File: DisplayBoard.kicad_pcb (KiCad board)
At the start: 4 copper layers, 35.6 x 38.1 mm, 42 parts, among them J201 Conn_Coaxial, J301 Conn_01x12_Pin, J401 Conn_01x04, Q301 L2N7002SLLT1G, U201 ESP32-S3-PICO-1-N8R2, U401 SN65HVD232, U501 USBLC6-2SC6, U502 AMS1117-3.3

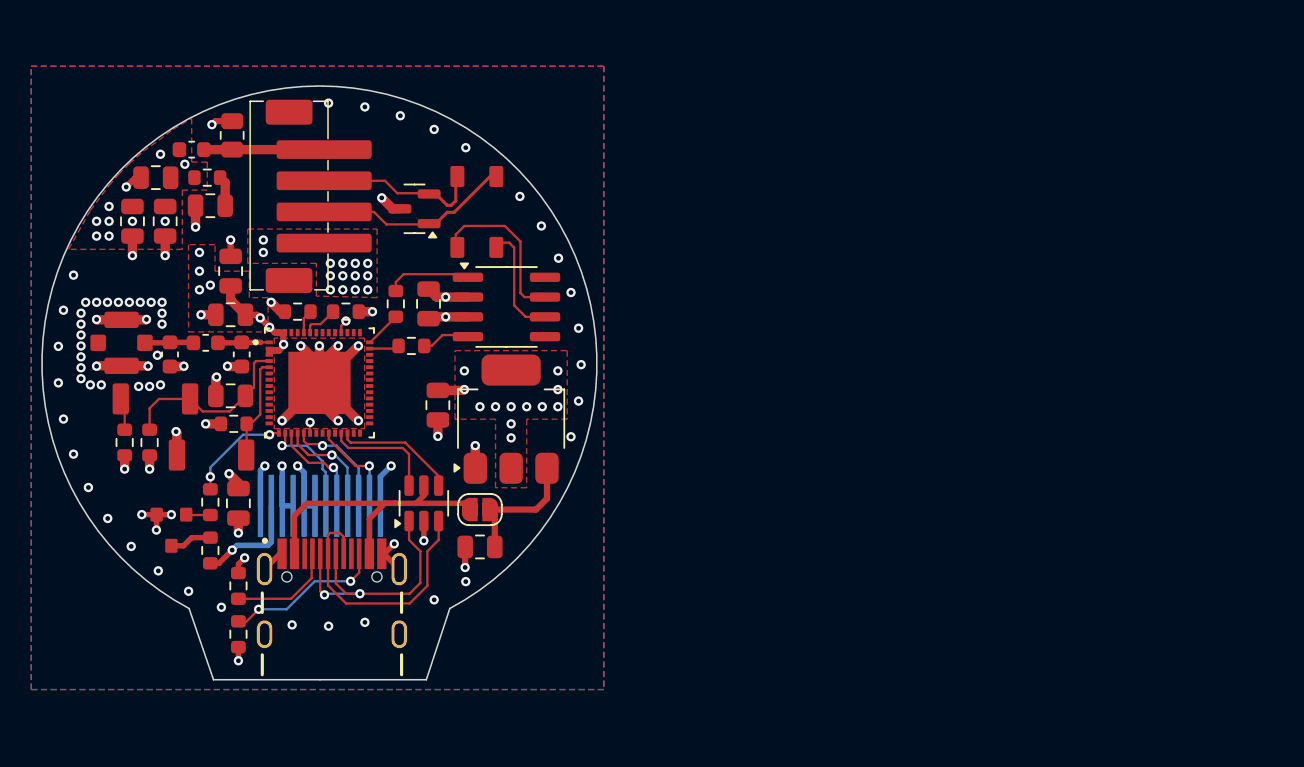
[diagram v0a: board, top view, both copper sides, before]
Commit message: Finished v1.1
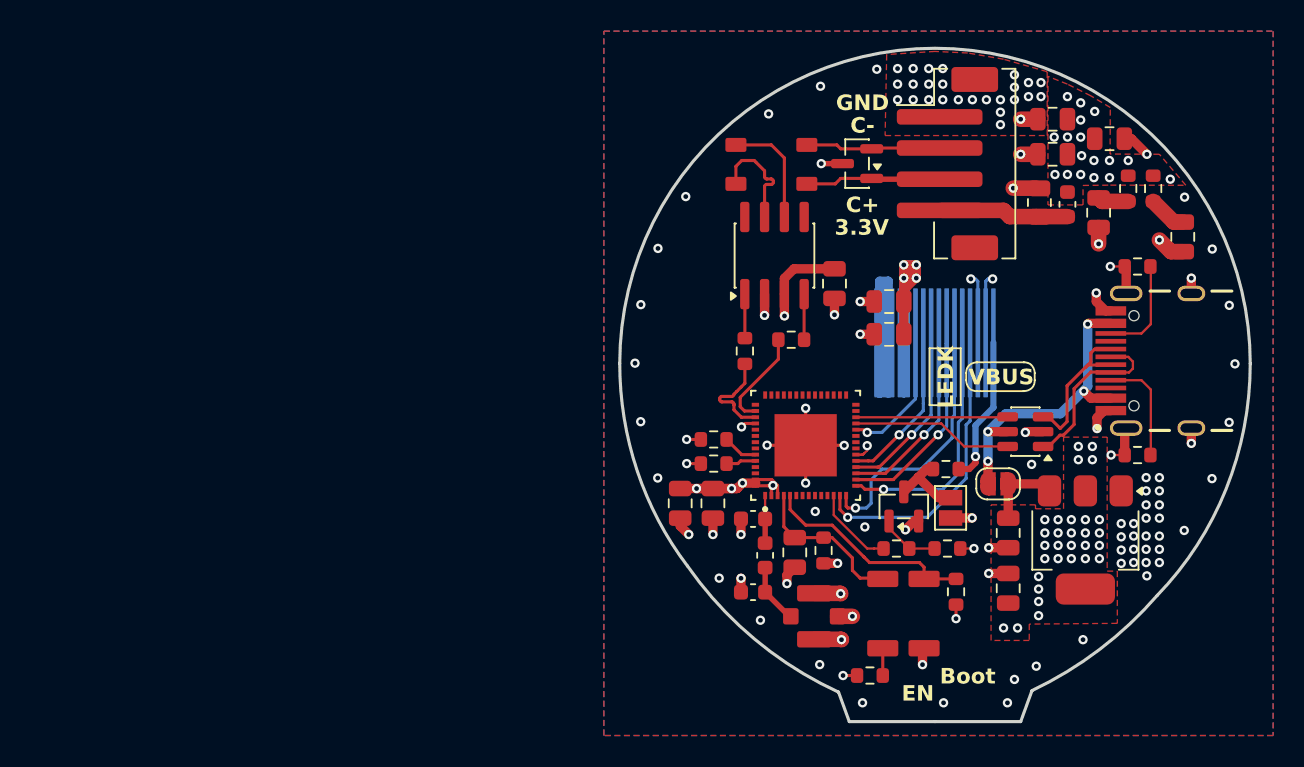
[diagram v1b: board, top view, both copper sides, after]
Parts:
- removed C201: 1uF, Capacitor_SMD:C_0805_2012Metric
- removed C202, C502: 22uF, Capacitor_SMD:C_0805_2012Metric
- removed C203: 0.1uF, Capacitor_SMD:C_0805_2012Metric
- removed C204, C205: 3.3pF, Capacitor_SMD:C_0603_1608Metric
- removed C301: 104, Capacitor_SMD:C_0805_2012Metric
- removed C401, C402: unkwn, Capacitor_SMD:C_0805_2012Metric
- removed C403, C405: 100nF, Capacitor_SMD:C_0805_2012Metric
- removed C404: 47uF, Capacitor_SMD:C_0805_2012Metric
- removed C501: 10uF, Capacitor_SMD:C_0805_2012Metric
- removed D401: SP4020-01FTG-C, Resistor_SMD:R_0805_2012Metric
- removed D402: PESD1CAN, Package_TO_SOT_SMD:SOT-23
- removed FB401: BLM18KG121TN1D, Inductor_SMD:L_0603_1608Metric
- removed J201: Conn_Coaxial, CustomFootprints:CONMHF1-SMD-G-T_U.FL
- removed J401: Conn_01x04, CustomFootprints:JST_PH_B4B_SM4_TB
- removed JP501: SolderJumper_2_Open, Jumper:SolderJumper-2_P1.3mm_Open_RoundedPad1.0x1.5mm
- removed L201: 2.2nH, Inductor_SMD:L_0603_1608Metric
- removed L401: TDK ACT45B-510-2P-TL003, CustomFootprints:TDK ACT45B-510-2P-TL003
- removed Q301: L2N7002SLLT1G, CustomFootprints:SOT_TO_92_L2N7002SLLT1G
- removed R201: 470, Resistor_SMD:R_0603_1608Metric
- removed R202, R203, R205, R206: 10k, Resistor_SMD:R_0603_1608Metric
- removed R204, R402: 100, Resistor_SMD:R_0603_1608Metric
- removed R301: 1k, Resistor_SMD:R_0603_1608Metric
- removed R302: 10, Resistor_SMD:R_0603_1608Metric
- removed R401: 3, Resistor_SMD:R_0603_1608Metric
- removed RST201: SW_SPST, CustomFootprints:XUNPU_Button
- removed Rusb501, Rusb502: 5.1k, Resistor_SMD:R_0603_1608Metric
- removed SPST201: BOOT, CustomFootprints:XUNPU_Button
- removed U201: ESP32-S3-PICO-1-N8R2, CustomFootprints:ESP32-S3-PICO-1
- removed U401: SN65HVD232, Package_SO:SOIC-8_3.9x4.9mm_P1.27mm
- removed U501: USBLC6-2SC6, Package_TO_SOT_SMD:SOT-23-6
- removed U502: AMS1117-3.3, Package_TO_SOT_SMD:SOT-223-3_TabPin2
- removed USBC501: USB4105-GF-A, CustomFootprints:USB-C_24P-2.0
- added C1: 1uF, Capacitor_SMD:C_0805_2012Metric, F.Cu at (130.5, 129.9)
- added C10: 100nF, Capacitor_SMD:C_0805_2012Metric, F.Cu at (147.1, 104.4)
- added C11: 47uF, Capacitor_SMD:C_0805_2012Metric, F.Cu at (150.0, 108.2)
- added C12: 47uF, Capacitor_SMD:C_0805_2012Metric, F.Cu at (155.4, 109.7)
- added C13: 100nF, Capacitor_SMD:C_0805_2012Metric, F.Cu at (133.1, 112.7)
- added C14: 10uF, Capacitor_SMD:C_0805_2012Metric, F.Cu at (144.2, 128.7)
- added C15: 22uF, Capacitor_SMD:C_0805_2012Metric, F.Cu at (144.2, 132.2)
- added C2: 22uF, Capacitor_SMD:C_0805_2012Metric, F.Cu at (123.2, 126.8)
- added C3: 100nF, Capacitor_SMD:C_0805_2012Metric, F.Cu at (125.2, 126.8)
- added C4: 3.3pF, Capacitor_SMD:C_0603_1608Metric, F.Cu at (127.8, 132.5)
- added C5: 3.3pF, Capacitor_SMD:C_0603_1608Metric, F.Cu at (127.8, 127.8)
- added C6: 100nF, Capacitor_SMD:C_0805_2012Metric, F.Cu at (136.6, 116.0)
- added C7: 100nF, Capacitor_SMD:C_0805_2012Metric, F.Cu at (136.6, 113.8)
- added C8: unkwn, Capacitor_SMD:C_0805_2012Metric, F.Cu at (147.1, 102.2)
- added C9: unkwn, Capacitor_SMD:C_0805_2012Metric, F.Cu at (150.7, 103.4)
- added D1: SP4020-01FTG-C, Resistor_SMD:R_0805_2012Metric, F.Cu at (146.2, 107.5)
- added D2: PESD1CAN, Package_TO_SOT_SMD:SOT-23, F.Cu at (134.5, 105.0)
- added FB1: BLM18KG121TN1D, Inductor_SMD:L_0603_1608Metric, F.Cu at (148.0, 107.6)
- added J1: Conn_Coaxial, CustomFootprints:CONMHF1-SMD-G-T_U.FL, F.Cu at (131.8, 134.1)
- added J3: Conn_01x04, Connector_JST:JST_PH_B4B-PH-SM4-TB_1x04-1MP_P2.00mm_Vertical, F.Cu at (140.3, 105.0)
- added JP1: SolderJumper_2_Open, Jumper:SolderJumper-2_P1.3mm_Open_Pad1.0x1.5mm, F.Cu at (140.5, 127.1)
- added JP2: SolderJumper_2_Open, Jumper:SolderJumper-2_P1.3mm_Open_RoundedPad1.0x1.5mm, F.Cu at (143.6, 125.5)
- added L1: 2.2nH, Inductor_SMD:L_0603_1608Metric, F.Cu at (128.6, 130.1)
- added L2: TDK ACT45B-510-2P-TL003, CustomFootprints:TDK ACT45B-510-2P-TL003, F.Cu at (129.0, 105.0)
- added Q1: Si2302CDS-T1-GE3, Package_TO_SOT_SMD:SOT-23, F.Cu at (137.5, 127.0)
- added R1: 470, Resistor_SMD:R_0603_1608Metric, F.Cu at (135.3, 137.8)
- added R10: 3, Resistor_SMD:R_0603_1608Metric, F.Cu at (151.9, 106.6)
- added R11: 3, Resistor_SMD:R_0603_1608Metric, F.Cu at (153.5, 106.6)
- added R12: 100, Resistor_SMD:R_0603_1608Metric, F.Cu at (130.3, 116.3)
- added R2: 10k, Resistor_SMD:R_0603_1608Metric, F.Cu at (140.8, 132.5)
- added R3: 10k, Resistor_SMD:R_0603_1608Metric, F.Cu at (132.3, 129.8)
- added R4: 100, Resistor_SMD:R_0603_1608Metric, F.Cu at (127.3, 117.0)
- added R5: 10k, Resistor_SMD:R_0603_1608Metric, F.Cu at (125.3, 122.7)
- added R6: 10k, Resistor_SMD:R_0603_1608Metric, F.Cu at (125.3, 124.2)
- added R7: 10k, Resistor_SMD:R_0603_1608Metric, F.Cu at (137.0, 129.7)
- added R8: 100k, Resistor_SMD:R_0603_1608Metric, F.Cu at (140.3, 129.7)
- added R9: 10, Resistor_SMD:R_0603_1608Metric, F.Cu at (140.2, 124.6)
- added RST1: SW_SPST, CustomFootprints:XUNPU_Button, F.Cu at (136.2, 136.1)
- added Rusb1: 5.1k, Resistor_SMD:R_0603_1608Metric, F.Cu at (152.5, 123.7)
- added Rusb2: 5.1k, Resistor_SMD:R_0603_1608Metric, F.Cu at (152.5, 111.6)
- added SPST1: BOOT, CustomFootprints:XUNPU_Button, F.Cu at (138.8, 136.1)
- added U1: ESP32-S3-PICO-1-N8R2, CustomFootprints:ESP32-S3-PICO-1, F.Cu at (131.2, 123.1)
- added U2: SN65HVD232, Package_SO:SOIC-8_3.9x4.9mm_P1.27mm, F.Cu at (129.2, 110.9)
- added U3: USBLC6-2SC6, Package_TO_SOT_SMD:SOT-23-6, F.Cu at (145.3, 122.2)
- added U4: AMS1117-3.3, Package_TO_SOT_SMD:SOT-223-3_TabPin2, F.Cu at (149.2, 129.2)
- added USBC1: USB4105-GF-A, CustomFootprints:USB-C_24P-2.0, F.Cu at (155.9, 117.7)
- J2: renamed from J301; value Conn_01x12_Pin -> Conn_01x16; footprint CustomFootprints:GC9A01_Connector -> CustomFootprints:ST77916
- moved J2 44.3 mm to (139.5, 116.5), turned to 180 degrees
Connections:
- J2 pad 1: GND -> LEDK
- J2 pad 10: /MCU/DIN -> /Display/IO0
- J2 pad 11: /MCU/RST -> /Display/TE
- J2 pad 12: GND -> +3.3V
- J2 pad 2: LEDK -> +3.3V
- J2 pad 3: +3.3V -> GND
- J2 pad 4: +3.3V -> /Display/CS
- J2 pad 5: GND -> /Display/CLK
- J2 pad 6: GND -> /Display/RST
- J2 pad 7: /MCU/DC -> /Display/IO3
- J2 pad 8: /MCU/CS -> /Display/IO2
- J2 pad 9: /MCU/CLK -> /Display/IO1
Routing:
- net +3.3V: track 19.8 -> 47.7 mm, vias 35 -> 61
- net /Display/CS: track 0.00 -> 19.0 mm, vias 0 -> 1
- net /Display/RST: track 0.00 -> 16.4 mm, vias 0 -> 1
- net /Display/CLK: track 0.00 -> 15.6 mm, vias 0 -> 1
- net /Display/IO3: track 0.00 -> 15.1 mm, vias 0 -> 1
- net /Display/IO2: track 0.00 -> 11.7 mm, vias 0 -> 1
- net CANH: track 11.0 -> 0.00 mm
- net /Display/IO1: track 0.00 -> 10.9 mm, vias 0 -> 1
- net /Display/IO0: track 0.00 -> 10.0 mm, vias 0 -> 1
- net /Display/TE: track 0.00 -> 8.39 mm, vias 0 -> 1
- net CANL: track 7.36 -> 0.00 mm
- net CAN-: track 0.00 -> 7.25 mm
- net CAN+: track 0.00 -> 7.22 mm
- net /MCU/DIN: track 7.18 -> 0.00 mm, vias 1 -> 0
- net /MCU/BOOT: track 6.66 -> 13.8 mm
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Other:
- board size 35.6 x 38.1 mm -> 40.5 x 43.2 mm
- board text added: "1"
- board text added: "3.3V"
- board text added: "Boot"
- board text added: "C+"
- board text added: "C-"
- board text added: "EN"
- board text added: "GND"
- board text added: "LEDK"
- board text added: "LEDK LEDA GND CS CLK RST IO3 IO2 IO1 IO0 TE TCC GND GND GND"
- board text added: "VBUS"
